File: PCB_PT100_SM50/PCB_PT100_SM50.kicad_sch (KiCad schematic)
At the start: 61 parts, among them U1 TPD4E1U06DBVR, U2 INA826AIDR, U3 TPS7A4901DGNT, U4 INA826AIDR, U5 OPA2188AIDR, U6 REF3012AIDBZR, U7 TPD4E1U06DBVR, U8 78L05 5V

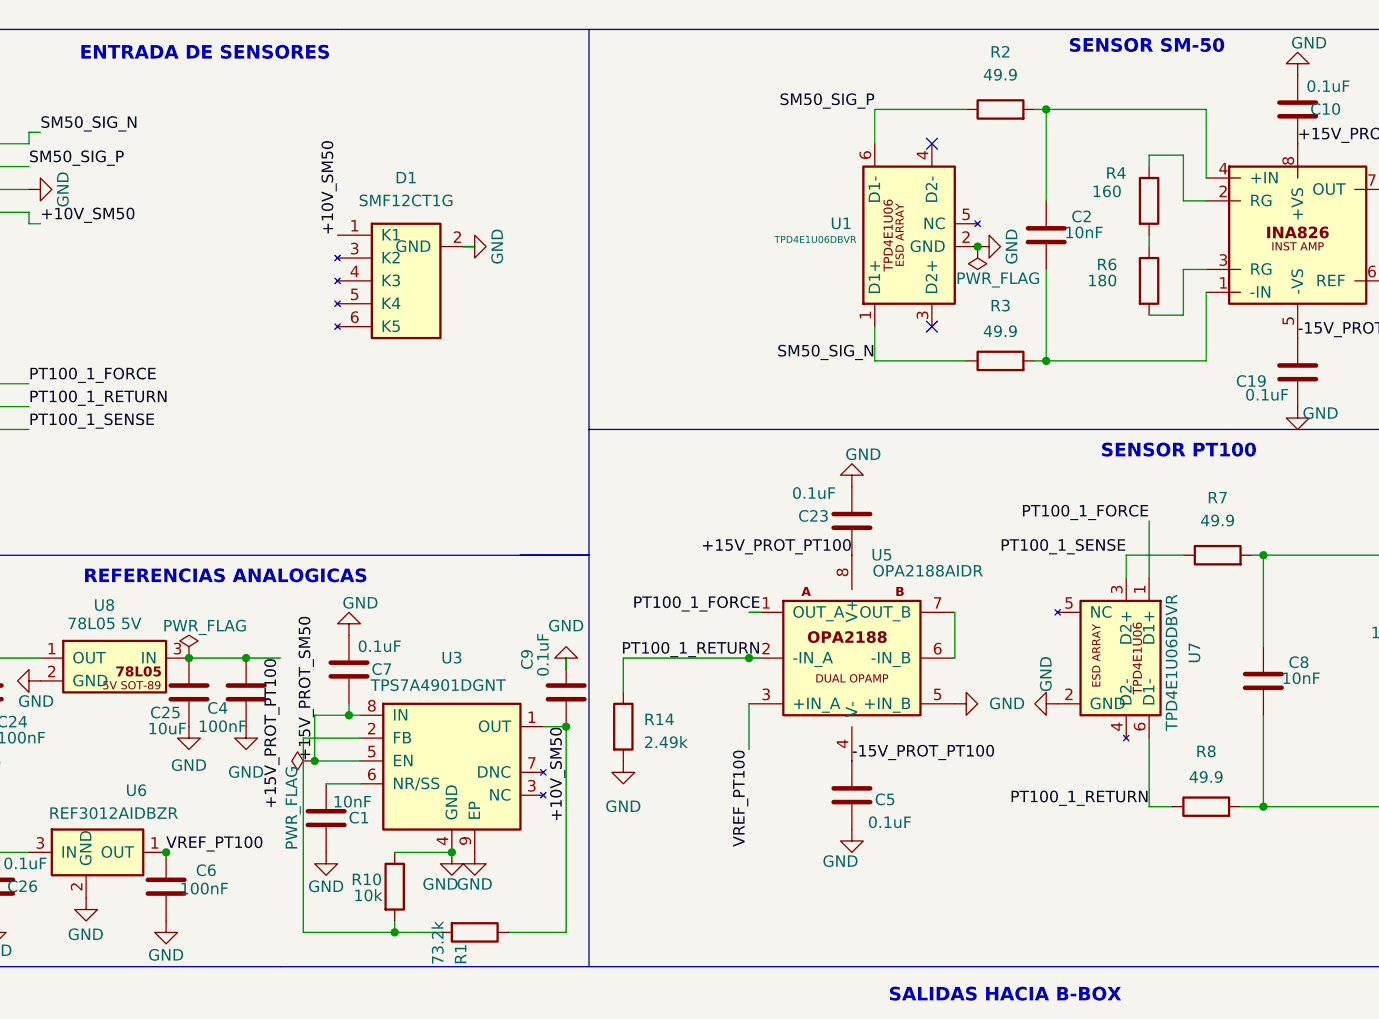
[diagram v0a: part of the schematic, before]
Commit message: Update LTspice schematics and fabrication outputs
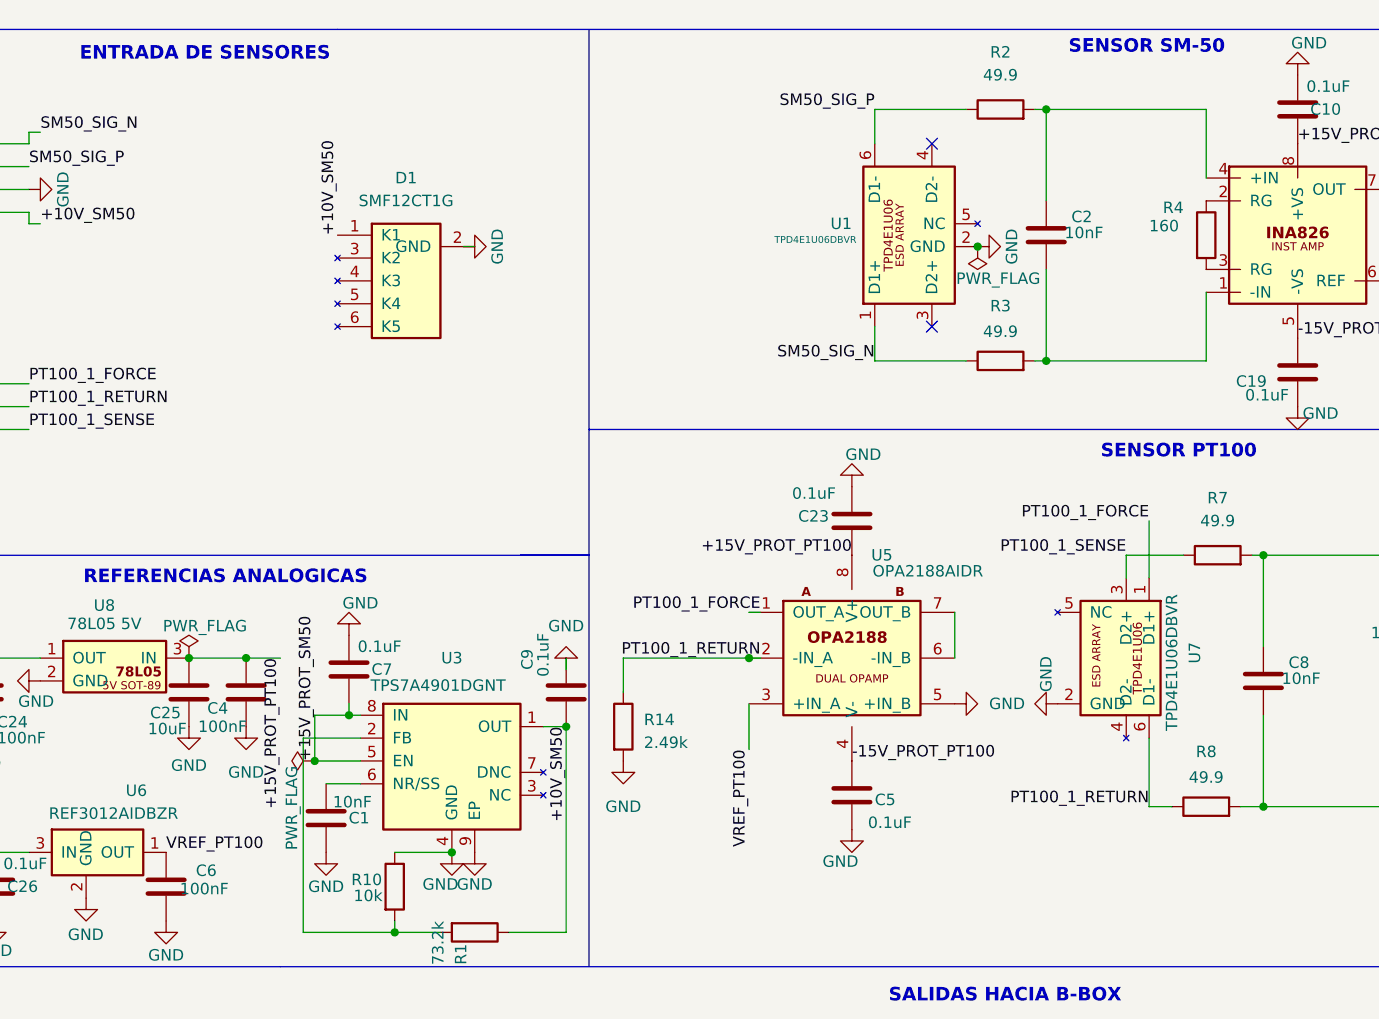
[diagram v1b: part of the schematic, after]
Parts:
- removed R6: 180, Resistor_SMD:R_0805_2012Metric, symbol Device:R
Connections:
- net at R4.2: now also U2.3 (RG)
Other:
- moved on the sheet: R4
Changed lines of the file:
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@@
 	)
 	(junction
-		(at 44.45 104.14)
-		(diameter 0)
-		(color 0 0 0 0)
-	)
-	(junction
 		(at 60.96 93.98)
 		(diameter 0)
@@
 	(wire
 		(pts
-			(xy 157.48 44.45) (xy 157.48 39.37)
-		)
-		(stroke
-			(width 0)
-			(type default)
-		)
-	)
-	(wire
-		(pts
 			(xy 35.56 130.81) (xy 43.18 130.81)
 		)
@@
 	(wire
 		(pts
-			(xy 153.67 36.83) (xy 153.67 35.56)
-		)
-		(stroke
-			(width 0)
-			(type default)
-		)
-	)
-	(wire
-		(pts
 			(xy 123.19 45.72) (xy 123.19 49.53)
 		)
@@
 	(wire
 		(pts
-			(xy 153.67 27.94) (xy 153.67 26.67)
-		)
-		(stroke
-			(width 0)
-			(type default)
-		)
-	)
-	(wire
-		(pts
 			(xy 29.21 25.4) (xy 24.13 25.4)
 		)
@@
 	(wire
 		(pts
-			(xy 157.48 26.67) (xy 157.48 31.75)
-		)
-		(stroke
-			(width 0)
-			(type default)
-		)
-	)
-	(wire
-		(pts
 			(xy 241.3 74.93) (xy 254 74.93)
 		)
@@
 	(wire
 		(pts
-			(xy 157.48 31.75) (xy 160.02 31.75)
-		)
-		(stroke
-			(width 0)
-			(type default)
-		)
-	)
-	(wire
-		(pts
 			(xy 254 30.48) (xy 266.7 30.48)
 		)
@@
 	(wire
 		(pts
-			(xy 153.67 44.45) (xy 157.48 44.45)
-		)
-		(stroke
-			(width 0)
-			(type default)
-		)
-	)
-	(wire
-		(pts
 			(xy 58.42 167.64) (xy 58.42 166.37)
 		)
@@
 	(wire
 		(pts
-			(xy 157.48 39.37) (xy 160.02 39.37)
-		)
-		(stroke
-			(width 0)
-			(type default)
-		)
-	)
-	(wire
-		(pts
-			(xy 153.67 26.67) (xy 157.48 26.67)
-		)
-		(stroke
-			(width 0)
-			(type default)
-		)
-	)
-	(wire
-		(pts
 			(xy 254 102.87) (xy 254 107.95)
 		)
@@
 	)
 	(symbol
-		(lib_id "Device:R")
-		(at 153.67 40.64 0)
-		(unit 1)
-		(exclude_from_sim no)
-		(in_bom yes)
-		(on_board yes)
-		(dnp no)
-		(property "Reference" "R6"
-			(at 147.828 38.862 0)
-			(effects
-				(font
-					(size 1.27 1.27)
-				)
-				(justify left)
-			)
-		)
-		(property "Value" "180"
-			(at 146.812 40.64 0)
-			(effects
-				(font
-					(size 1.27 1.27)
-				)
-				(justify left)
-			)
-		)
-		(property "Footprint" "Resistor_SMD:R_0805_2012Metric"
-			(at 151.892 40.64 90)
-			(effects
-				(font
-					(size 1.27 1.27)
-				)
-				(hide yes)
-			)
-		)
-		(property "Datasheet" "~"
-			(at 153.67 40.64 0)
-			(effects
-				(font
-					(size 1.27 1.27)
-				)
-				(hide yes)
-			)
-		)
-		(property "Description" "Resistor"
-			(at 153.67 40.64 0)
-			(effects
-				(font
-					(size 1.27 1.27)
-				)
-				(hide yes)
-			)
-		)
-		(pin "2"
-		)
-		(pin "1"
-		)
-		(instances
-			(project "PCB_PT100_SM50"
-				(path "/07ccf049-058a-470e-ab5d-8d6ecbc88c08"
-					(reference "R6")
-					(unit 1)
-				)
-			)
-		)
-	)
-	(symbol
 		(lib_id "power:GND")
 		(at 24.13 90.17 0)
@@
 	(symbol
 		(lib_id "Device:R")
-		(at 153.67 31.75 0)
+		(at 160.02 35.56 0)
 		(unit 1)
 		(exclude_from_sim no)
@@
 		(dnp no)
 		(property "Reference" "R4"
-			(at 148.844 28.702 0)
+			(at 155.194 32.512 0)
 			(effects
 				(font
@@
 		)
 		(property "Value" "160"
-			(at 147.32 30.734 0)
+			(at 153.67 34.544 0)
 			(effects
 				(font
@@
 		)
 		(property "Footprint" "Resistor_SMD:R_0805_2012Metric"
-			(at 151.892 31.75 90)
+			(at 158.242 35.56 90)
 			(effects
 				(font
@@
 		)
 		(property "Datasheet" "~"
-			(at 153.67 31.75 0)
+			(at 160.02 35.56 0)
 			(effects
 				(font
@@
 		)
 		(property "Description" "Resistor"
-			(at 153.67 31.75 0)
+			(at 160.02 35.56 0)
 			(effects
 				(font

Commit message: Restaurar version SM-50 0-5V
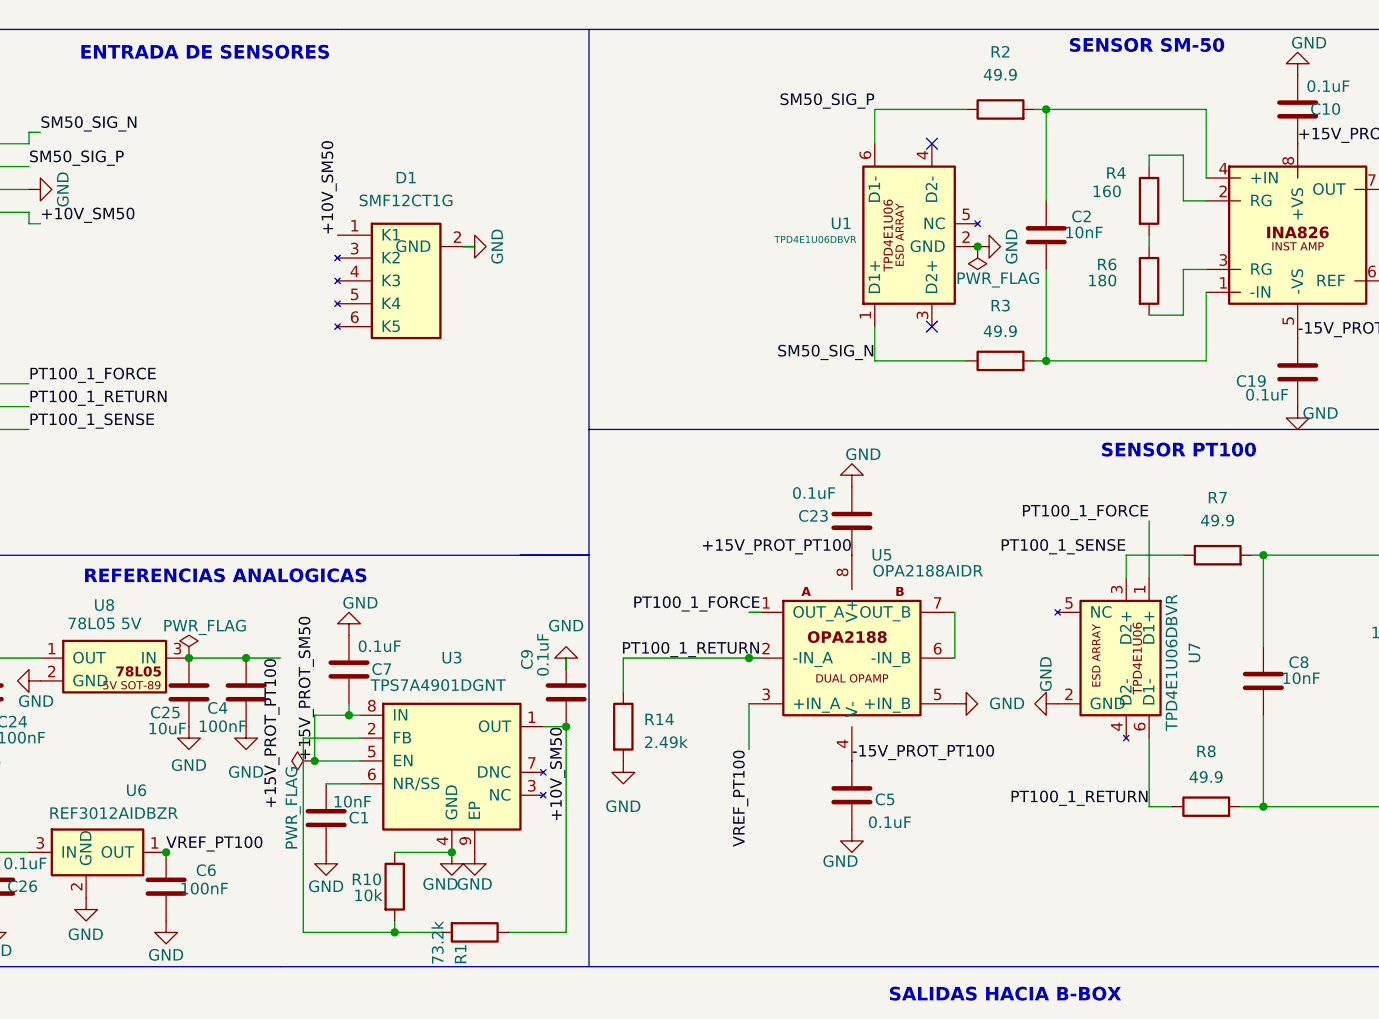
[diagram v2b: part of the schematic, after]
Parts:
- added R6: 180, Resistor_SMD:R_0805_2012Metric, symbol Device:R
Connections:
- net at R4.2: now also R6.1; no longer U2.3 (RG)
- new net: R6.2, U2.3 (RG)
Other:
- moved on the sheet: R4
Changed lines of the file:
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@@
 	)
 	(junction
+		(at 44.45 104.14)
+		(diameter 0)
+		(color 0 0 0 0)
+	)
+	(junction
 		(at 60.96 93.98)
 		(diameter 0)
@@
 	(wire
 		(pts
+			(xy 157.48 44.45) (xy 157.48 39.37)
+		)
+		(stroke
+			(width 0)
+			(type default)
+		)
+	)
+	(wire
+		(pts
 			(xy 35.56 130.81) (xy 43.18 130.81)
 		)
@@
 	(wire
 		(pts
+			(xy 153.67 36.83) (xy 153.67 35.56)
+		)
+		(stroke
+			(width 0)
+			(type default)
+		)
+	)
+	(wire
+		(pts
 			(xy 123.19 45.72) (xy 123.19 49.53)
 		)
@@
 	(wire
 		(pts
+			(xy 153.67 27.94) (xy 153.67 26.67)
+		)
+		(stroke
+			(width 0)
+			(type default)
+		)
+	)
+	(wire
+		(pts
 			(xy 29.21 25.4) (xy 24.13 25.4)
 		)
@@
 	(wire
 		(pts
+			(xy 157.48 26.67) (xy 157.48 31.75)
+		)
+		(stroke
+			(width 0)
+			(type default)
+		)
+	)
+	(wire
+		(pts
 			(xy 241.3 74.93) (xy 254 74.93)
 		)
@@
 	(wire
 		(pts
+			(xy 157.48 31.75) (xy 160.02 31.75)
+		)
+		(stroke
+			(width 0)
+			(type default)
+		)
+	)
+	(wire
+		(pts
 			(xy 254 30.48) (xy 266.7 30.48)
 		)
@@
 	(wire
 		(pts
+			(xy 153.67 44.45) (xy 157.48 44.45)
+		)
+		(stroke
+			(width 0)
+			(type default)
+		)
+	)
+	(wire
+		(pts
 			(xy 58.42 167.64) (xy 58.42 166.37)
 		)
@@
 	(wire
 		(pts
+			(xy 157.48 39.37) (xy 160.02 39.37)
+		)
+		(stroke
+			(width 0)
+			(type default)
+		)
+	)
+	(wire
+		(pts
+			(xy 153.67 26.67) (xy 157.48 26.67)
+		)
+		(stroke
+			(width 0)
+			(type default)
+		)
+	)
+	(wire
+		(pts
 			(xy 254 102.87) (xy 254 107.95)
 		)
@@
 	)
 	(symbol
+		(lib_id "Device:R")
+		(at 153.67 40.64 0)
+		(unit 1)
+		(exclude_from_sim no)
+		(in_bom yes)
+		(on_board yes)
+		(dnp no)
+		(property "Reference" "R6"
+			(at 147.828 38.862 0)
+			(effects
+				(font
+					(size 1.27 1.27)
+				)
+				(justify left)
+			)
+		)
+		(property "Value" "180"
+			(at 146.812 40.64 0)
+			(effects
+				(font
+					(size 1.27 1.27)
+				)
+				(justify left)
+			)
+		)
+		(property "Footprint" "Resistor_SMD:R_0805_2012Metric"
+			(at 151.892 40.64 90)
+			(effects
+				(font
+					(size 1.27 1.27)
+				)
+				(hide yes)
+			)
+		)
+		(property "Datasheet" "~"
+			(at 153.67 40.64 0)
+			(effects
+				(font
+					(size 1.27 1.27)
+				)
+				(hide yes)
+			)
+		)
+		(property "Description" "Resistor"
+			(at 153.67 40.64 0)
+			(effects
+				(font
+					(size 1.27 1.27)
+				)
+				(hide yes)
+			)
+		)
+		(pin "2"
+		)
+		(pin "1"
+		)
+		(instances
+			(project "PCB_PT100_SM50"
+				(path "/07ccf049-058a-470e-ab5d-8d6ecbc88c08"
+					(reference "R6")
+					(unit 1)
+				)
+			)
+		)
+	)
+	(symbol
 		(lib_id "power:GND")
 		(at 24.13 90.17 0)
@@
 	(symbol
 		(lib_id "Device:R")
-		(at 160.02 35.56 0)
+		(at 153.67 31.75 0)
 		(unit 1)
 		(exclude_from_sim no)
@@
 		(dnp no)
 		(property "Reference" "R4"
-			(at 155.194 32.512 0)
+			(at 148.844 28.702 0)
 			(effects
 				(font
@@
 		)
 		(property "Value" "160"
-			(at 153.67 34.544 0)
+			(at 147.32 30.734 0)
 			(effects
 				(font
@@
 		)
 		(property "Footprint" "Resistor_SMD:R_0805_2012Metric"
-			(at 158.242 35.56 90)
+			(at 151.892 31.75 90)
 			(effects
 				(font
@@
 		)
 		(property "Datasheet" "~"
-			(at 160.02 35.56 0)
+			(at 153.67 31.75 0)
 			(effects
 				(font
@@
 		)
 		(property "Description" "Resistor"
-			(at 160.02 35.56 0)
+			(at 153.67 31.75 0)
 			(effects
 				(font
